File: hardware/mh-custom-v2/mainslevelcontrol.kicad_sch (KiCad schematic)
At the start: 0 parts

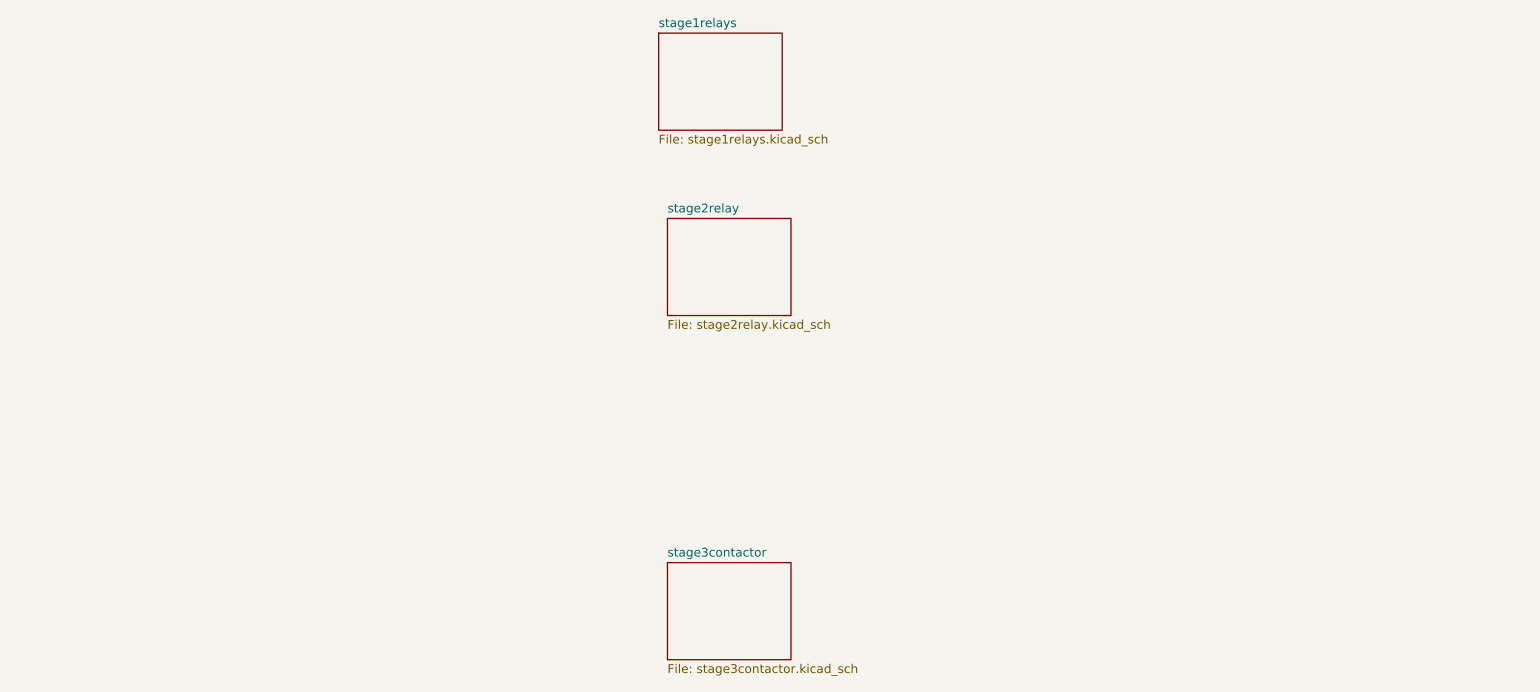
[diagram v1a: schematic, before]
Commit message: just ordered from JLCPCB
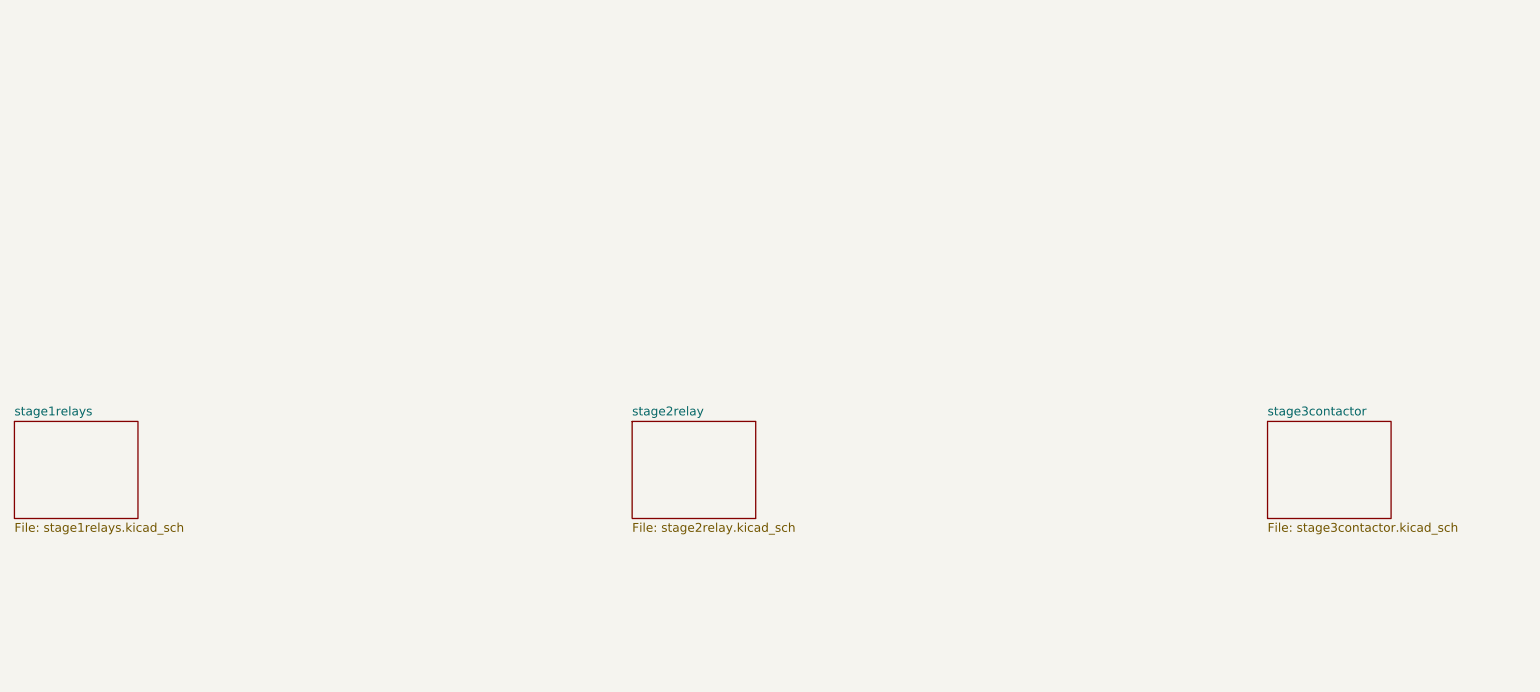
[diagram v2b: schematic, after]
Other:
- company: (none) -> Corey Rice & MakeHaven
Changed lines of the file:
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@@
 (kicad_sch (version 20211123) (generator eeschema)
   (paper "A4")
-  (sheet (at 137.16 140.97) (size 17.78 13.97) (fields_autoplaced)
+  (title_block
+    (date "2022-10-09")
+    (rev "2")
+    (company "Corey Rice & MakeHaven")
+  )
+  (sheet (at 223.52 120.65) (size 17.78 13.97) (fields_autoplaced)
     (stroke (width 0.1524) (type solid) (color 0 0 0 0))
     (fill (color 0 0 0 0.0000))
-    (property "Sheet name" "stage3contactor" (id 0) (at 137.16 140.2584 0)
+    (property "Sheet name" "stage3contactor" (id 0) (at 223.52 119.9384 0)
       (effects (font (size 1.27 1.27)) (justify left bottom))
     )
-    (property "Sheet file" "stage3contactor.kicad_sch" (id 1) (at 137.16 155.5246 0)
+    (property "Sheet file" "stage3contactor.kicad_sch" (id 1) (at 223.52 135.2046 0)
       (effects (font (size 1.27 1.27)) (justify left top))
     )
   )
-  (sheet (at 135.89 64.77) (size 17.78 13.97) (fields_autoplaced)
+  (sheet (at 43.18 120.65) (size 17.78 13.97) (fields_autoplaced)
     (stroke (width 0.1524) (type solid) (color 0 0 0 0))
     (fill (color 0 0 0 0.0000))
-    (property "Sheet name" "stage1relays" (id 0) (at 135.89 64.0584 0)
+    (property "Sheet name" "stage1relays" (id 0) (at 43.18 119.9384 0)
       (effects (font (size 1.27 1.27)) (justify left bottom))
     )
-    (property "Sheet file" "stage1relays.kicad_sch" (id 1) (at 135.89 79.3246 0)
+    (property "Sheet file" "stage1relays.kicad_sch" (id 1) (at 43.18 135.2046 0)
       (effects (font (size 1.27 1.27)) (justify left top))
     )
   )
-  (sheet (at 137.16 91.44) (size 17.78 13.97) (fields_autoplaced)
+  (sheet (at 132.08 120.65) (size 17.78 13.97) (fields_autoplaced)
     (stroke (width 0.1524) (type solid) (color 0 0 0 0))
     (fill (color 0 0 0 0.0000))
-    (property "Sheet name" "stage2relay" (id 0) (at 137.16 90.7284 0)
+    (property "Sheet name" "stage2relay" (id 0) (at 132.08 119.9384 0)
       (effects (font (size 1.27 1.27)) (justify left bottom))
     )
-    (property "Sheet file" "stage2relay.kicad_sch" (id 1) (at 137.16 105.9946 0)
+    (property "Sheet file" "stage2relay.kicad_sch" (id 1) (at 132.08 135.2046 0)
       (effects (font (size 1.27 1.27)) (justify left top))
     )
